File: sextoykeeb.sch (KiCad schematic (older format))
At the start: 66 parts, among them J1 Conn_01x06, J2 Conn_01x06, SW1 SW_Push, SW2 SW_Push, SW3 SW_Push, SW4 SW_Push, SW5 SW_Push, SW6 SW_Push, SW7 SW_Push, SW8 SW_Push, SW9 SW_Push, U1 nRF52840_holyiot_18010, U2 MCP1700-3302E_SOT23, U3 TP4056, U4 SRV05-4, U5 FS8205, U6 DW01A

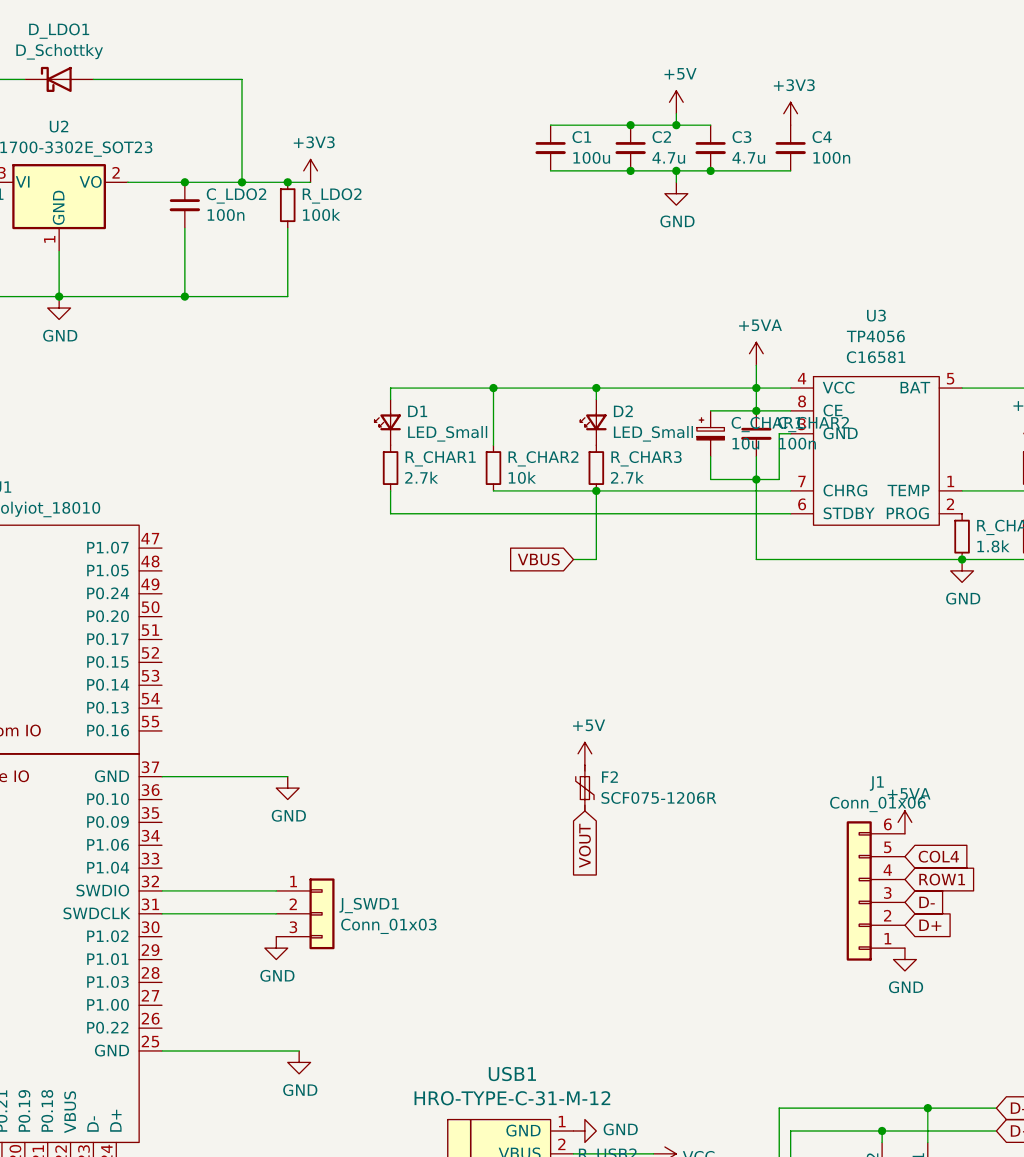
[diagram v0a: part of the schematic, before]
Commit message: finished pcb for real this time
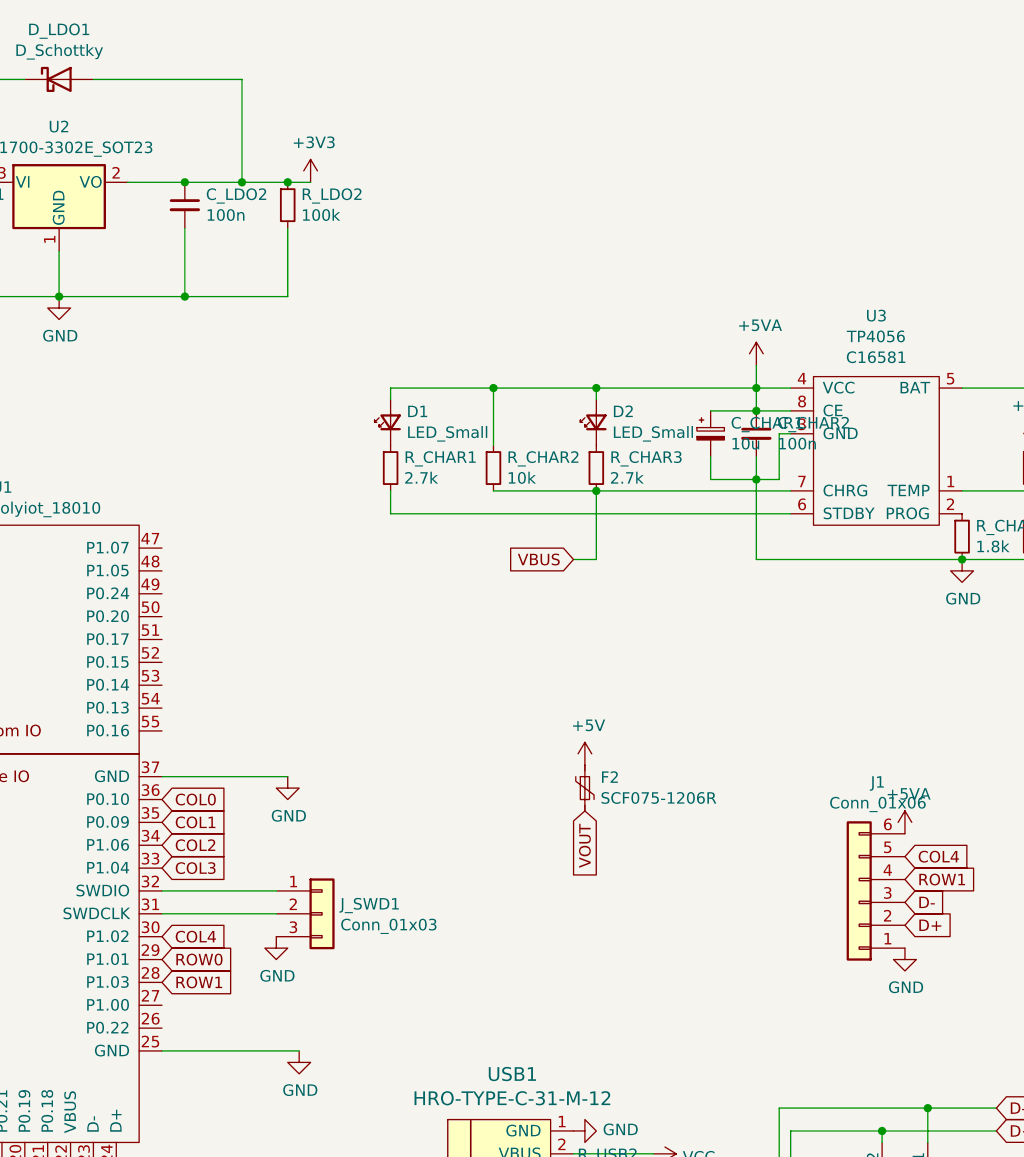
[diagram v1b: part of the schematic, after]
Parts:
- removed C1: 100u, Capacitor_SMD:C_0603_1608Metric_Pad1.08x0.95mm_HandSolder, symbol Device:C_Small
- removed C2, C3: 4.7u, Capacitor_SMD:C_0603_1608Metric_Pad1.08x0.95mm_HandSolder, symbol Device:C_Small
- removed C4: 100n, Capacitor_SMD:C_0603_1608Metric_Pad1.08x0.95mm_HandSolder, symbol Device:C_Small
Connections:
- net COL0: now also U1.36 (P0.10)
- net COL1: now also U1.35 (P0.09)
- net COL2: now also U1.34 (P1.06)
- net COL3: now also U1.33 (P1.04)
- net COL4: now also U1.30 (P1.02)
- net ROW0: now also U1.29 (P1.01)
- net ROW1: now also U1.28 (P1.03)
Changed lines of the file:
@@
 	1    0    0    -1
 $EndComp
-$Comp
-L Device:C_Small C1
-U 1 1 5FD2A2F2
-P 5250 1350
-F 0 "C1" H 5342 1396 50  0000 L CNN
-F 1 "100u" H 5342 1305 50  0000 L CNN
-F 2 "Capacitor_SMD:C_0603_1608Metric_Pad1.08x0.95mm_HandSolder" H 5250 1350 50  0001 C CNN
-F 3 "~" H 5250 1350 50  0001 C CNN
-	1    5250 1350
-	1    0    0    -1
-$EndComp
-$Comp
-L Device:C_Small C2
-U 1 1 5FD2AADB
-P 5600 1350
-F 0 "C2" H 5692 1396 50  0000 L CNN
-F 1 "4.7u" H 5692 1305 50  0000 L CNN
-F 2 "Capacitor_SMD:C_0603_1608Metric_Pad1.08x0.95mm_HandSolder" H 5600 1350 50  0001 C CNN
-F 3 "~" H 5600 1350 50  0001 C CNN
-	1    5600 1350
-	1    0    0    -1
-$EndComp
-$Comp
-L Device:C_Small C3
-U 1 1 5FD2B2F1
-P 5950 1350
-F 0 "C3" H 6042 1396 50  0000 L CNN
-F 1 "4.7u" H 6042 1305 50  0000 L CNN
-F 2 "Capacitor_SMD:C_0603_1608Metric_Pad1.08x0.95mm_HandSolder" H 5950 1350 50  0001 C CNN
-F 3 "~" H 5950 1350 50  0001 C CNN
-	1    5950 1350
-	1    0    0    -1
-$EndComp
-$Comp
-L Device:C_Small C4
-U 1 1 5FD2B854
-P 6300 1350
-F 0 "C4" H 6392 1396 50  0000 L CNN
-F 1 "100n" H 6392 1305 50  0000 L CNN
-F 2 "Capacitor_SMD:C_0603_1608Metric_Pad1.08x0.95mm_HandSolder" H 6300 1350 50  0001 C CNN
-F 3 "~" H 6300 1350 50  0001 C CNN
-	1    6300 1350
-	1    0    0    -1
-$EndComp
-$Comp
-L power:+3V3 #PWR0128
-U 1 1 5FD2ECEE
-P 6300 1250
-F 0 "#PWR0128" H 6300 1100 50  0001 C CNN
-F 1 "+3V3" H 6315 1423 50  0000 C CNN
-F 2 "" H 6300 1250 50  0001 C CNN
-F 3 "" H 6300 1250 50  0001 C CNN
-	1    6300 1250
-	1    0    0    -1
-$EndComp
-$Comp
-L power:GND #PWR0129
-U 1 1 5FD2EFCD
-P 5800 1500
-F 0 "#PWR0129" H 5800 1250 50  0001 C CNN
-F 1 "GND" H 5805 1327 50  0000 C CNN
-F 2 "" H 5800 1500 50  0001 C CNN
-F 3 "" H 5800 1500 50  0001 C CNN
-	1    5800 1500
-	1    0    0    -1
-$EndComp
-$Comp
-L power:+5V #PWR0130
-U 1 1 5FD30984
-P 5800 1200
-F 0 "#PWR0130" H 5800 1050 50  0001 C CNN
-F 1 "+5V" H 5815 1373 50  0000 C CNN
-F 2 "" H 5800 1200 50  0001 C CNN
-F 3 "" H 5800 1200 50  0001 C CNN
-	1    5800 1200
-	1    0    0    -1
-$EndComp
-Wire Wire Line
-	5250 1250 5600 1250
-Connection ~ 5600 1250
-Wire Wire Line
-	5600 1250 5800 1250
-Wire Wire Line
-	5800 1200 5800 1250
-Connection ~ 5800 1250
-Wire Wire Line
-	5800 1250 5950 1250
-Wire Wire Line
-	5250 1450 5600 1450
-Connection ~ 5600 1450
-Wire Wire Line
-	5600 1450 5800 1450
-Connection ~ 5950 1450
-Wire Wire Line
-	5950 1450 6300 1450
-Wire Wire Line
-	5800 1450 5800 1500
-Connection ~ 5800 1450
-Wire Wire Line
-	5800 1450 5950 1450
 Text GLabel 6800 4750 2    50   Input ~ 0
 D+
@@
 Text GLabel 10900 3750 1    50   Input ~ 0
 COL3
+Text GLabel 3550 4200 2    50   Input ~ 0
+COL0
+Text GLabel 3550 4300 2    50   Input ~ 0
+COL1
+Text GLabel 3550 4400 2    50   Input ~ 0
+COL2
+Text GLabel 3550 4500 2    50   Input ~ 0
+COL3
+Text GLabel 3550 4800 2    50   Input ~ 0
+COL4
+Text GLabel 3550 4900 2    50   Input ~ 0
+ROW0
+Text GLabel 3550 5000 2    50   Input ~ 0
+ROW1
 $EndSCHEMATC

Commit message: switched to 'Taylor spacing', moved most of the components, reversible switch footprints
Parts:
- SW_CHAR1: footprint kicad-keyboard-parts:ESP3020 -> kicad-keyboard-parts-linux:ESP3020
- U1: footprint kicad-keyboard-parts:nRF52840_holyiot_18010 -> kicad-keyboard-parts-linux:nRF52840_holyiot_18010; symbol kicad-keyboard-parts:nRF52840_holyiot_18010 -> sextoykeeb-rescue:nRF52840_holyiot_18010-kicad-keyboard-parts
- U3: symbol kicad-keyboard-parts:TP4056 -> sextoykeeb-rescue:TP4056-kicad-keyboard-parts
- U5: symbol kicad-keyboard-parts:FS8205 -> sextoykeeb-rescue:FS8205-kicad-keyboard-parts
- U6: symbol kicad-keyboard-parts:DW01A -> sextoykeeb-rescue:DW01A-kicad-keyboard-parts
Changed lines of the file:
@@
 $EndDescr
 $Comp
-L kicad-keyboard-parts:nRF52840_holyiot_18010 U1
+L sextoykeeb-rescue:nRF52840_holyiot_18010-kicad-keyboard-parts U1
 U 1 1 5FBA5D39
 P 2850 4350
 F 0 "U1" H 2850 5865 50  0000 C CNN
 F 1 "nRF52840_holyiot_18010" H 2850 5774 50  0000 C CNN
-F 2 "kicad-keyboard-parts:nRF52840_holyiot_18010" H 2950 4750 50  0001 C CNN
+F 2 "kicad-keyboard-parts-linux:nRF52840_holyiot_18010" H 2950 4750 50  0001 C CNN
 F 3 "http://www.holyiot.com/tp/2019042516322180424.pdf" H 2950 4750 50  0001 C CNN
 	1    2850 4350
@@
 $EndComp
 $Comp
-L kicad-keyboard-parts:TP4056 U3
+L sextoykeeb-rescue:TP4056-kicad-keyboard-parts U3
 U 1 1 5FC45463
 P 6700 2650
@@
 F 0 "SW_CHAR1" H 8150 1775 50  0000 C CNN
 F 1 "SW_SPDT" H 8150 1866 50  0000 C CNN
-F 2 "kicad-keyboard-parts:ESP3020" H 8150 2100 50  0001 C CNN
+F 2 "kicad-keyboard-parts-linux:ESP3020" H 8150 2100 50  0001 C CNN
 F 3 "~" H 8150 2100 50  0001 C CNN
 	1    8150 2100
@@
 $EndComp
 $Comp
-L kicad-keyboard-parts:FS8205 U5
+L sextoykeeb-rescue:FS8205-kicad-keyboard-parts U5
 U 1 1 5FCBCA45
 P 9550 2950
@@
 $EndComp
 $Comp
-L kicad-keyboard-parts:DW01A U6
+L sextoykeeb-rescue:DW01A-kicad-keyboard-parts U6
 U 1 1 5FCC0E92
 P 10350 2500
